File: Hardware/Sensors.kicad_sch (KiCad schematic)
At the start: 0 parts

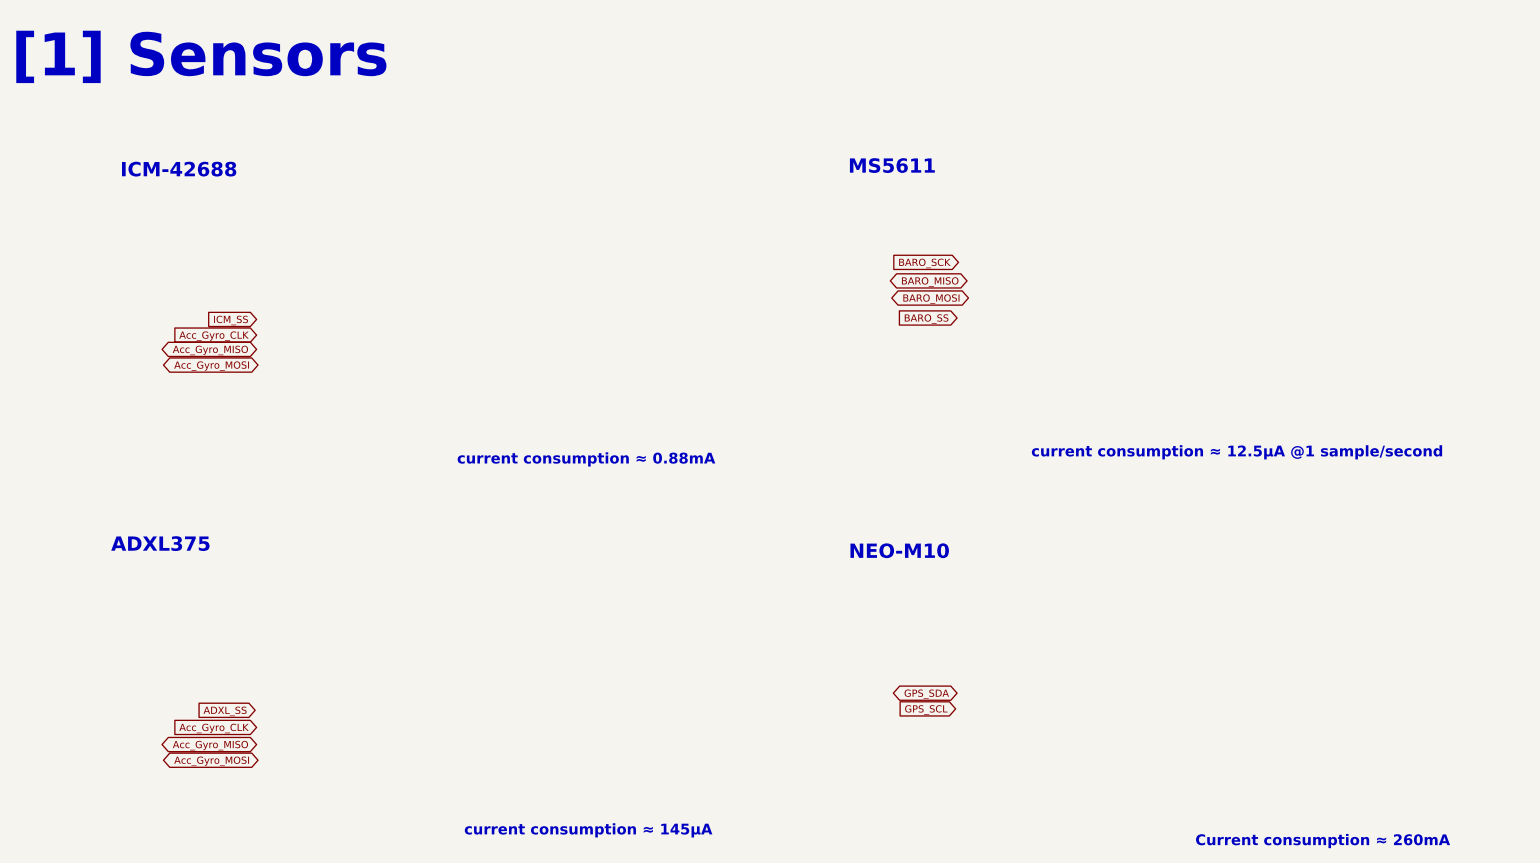
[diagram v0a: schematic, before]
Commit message: Updated schematics
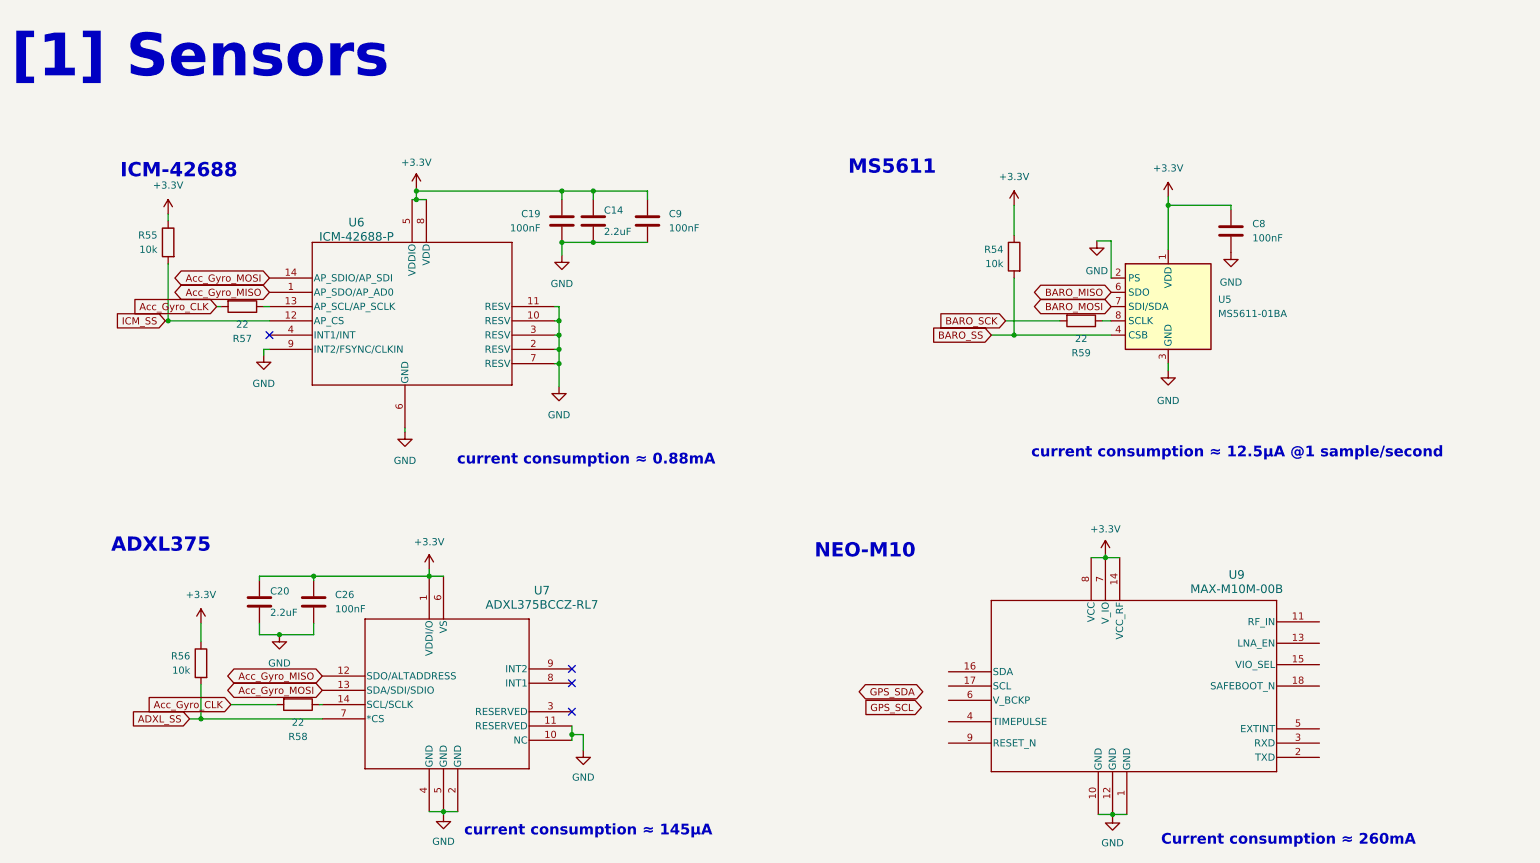
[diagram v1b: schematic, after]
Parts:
- added C14, C20: 2.2uF, Capacitor_SMD:C_0402_1005Metric, symbol Device:C
- added C19, C26, C8, C9: 100nF, Capacitor_SMD:C_0402_1005Metric, symbol Device:C
- added R54, R55, R56: 10k, Resistor_SMD:R_0402_1005Metric, symbol Device:R
- added R57, R58, R59: 22, Resistor_SMD:R_0402_1005Metric, symbol Device:R
- added U5: MS5611-01BA, Package_LGA:LGA-8_3x5mm_P1.25mm, symbol Sensor_Pressure:MS5611-01BA
- added U6: ICM-42688-P, LGA14_2P5X3X0P91_TDK, symbol 2026-06-16_08-50-59:ICM-42688-P
- added U7: ADXL375BCCZ-RL7, ADXL375BCCZ_RL7:LGA_CC-14-1_ADI, symbol 2026-07-20_16-43-50:ADXL375BCCZ-RL7
- added U9: MAX-M10M-00B, MAX_M10M_00B:MOD18_MAX-M10M_UBL, symbol 2026-07-20_17-18-28:MAX-M10M-00B
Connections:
- net ADXL_SS: now also R56.2, U7.7 (*CS)
- net Acc_Gyro_CLK: now also R57.2, R58.2
- net Acc_Gyro_MISO: now also U6.1 (AP_SDO/AP_AD0), U7.12 (SDO/ALTADDRESS)
- net Acc_Gyro_MOSI: now also U6.14 (AP_SDIO/AP_SDI), U7.13 (SDA/SDI/SDIO)
- net BARO_MISO: now also U5.6 (SDO)
- net BARO_MOSI: now also U5.7 (SDI/SDA)
- net BARO_SCK: now also R59.2
- net BARO_SS: now also R54.2, U5.4 (CSB), U5.5 (CSB)
- net ICM_SS: now also R55.2, U6.12 (AP_CS)
- new net: R59.1, U5.8 (SCLK)
- new net: R58.1, U7.14 (SCL/SCLK)
- new net: R57.1, U6.13 (AP_SCL/AP_SCLK)
- new net +3.3V: C14.1, C19.1, C20.1, C26.1, C8.1, C9.1, R54.1, R55.1, R56.1, U5.1 (VDD), U6.5 (VDDIO), U6.8 (VDD), U7.1 (VDDI/O), U7.6 (VS), U9.14 (VCC_RF), U9.7 (V_IO), U9.8 (VCC)
- new net GND: C14.2, C19.2, C20.2, C26.2, C8.2, C9.2, U5.2 (PS), U5.3 (GND), U6.10 (RESV), U6.11 (RESV), U6.2 (RESV), U6.3 (RESV), U6.6 (GND), U6.7 (RESV), U6.9 (INT2/FSYNC/CLKIN), U7.10 (NC), U7.11 (RESERVED), U7.2 (GND), U7.4 (GND), U7.5 (GND), U9.1 (GND), U9.10 (GND), U9.12 (GND)
- no-connect marks 0 -> 4
